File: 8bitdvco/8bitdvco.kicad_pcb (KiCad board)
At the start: 2 copper layers, 87.4 x 66.8 mm, 30 parts, among them J1 PWR_IN, J2 SPI, J3 DISP, J4 UART, J5 THERM, J6 FAN, J7 HEAT, SW1 SW_RST, SW2 SW_STOP_MODE, SW3 SW_START_SET, U1 ATmega328P-PU, Y1 16MHz

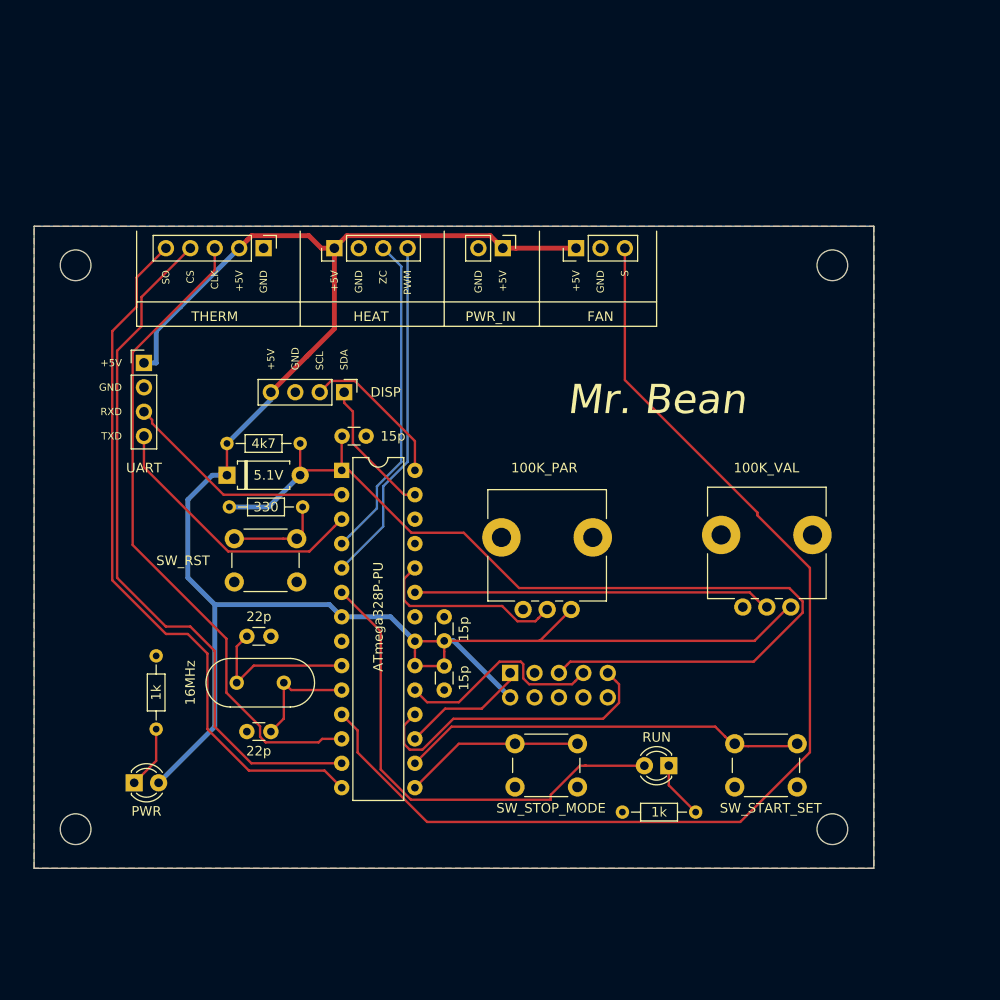
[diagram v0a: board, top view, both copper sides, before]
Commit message: done without errors and warnings
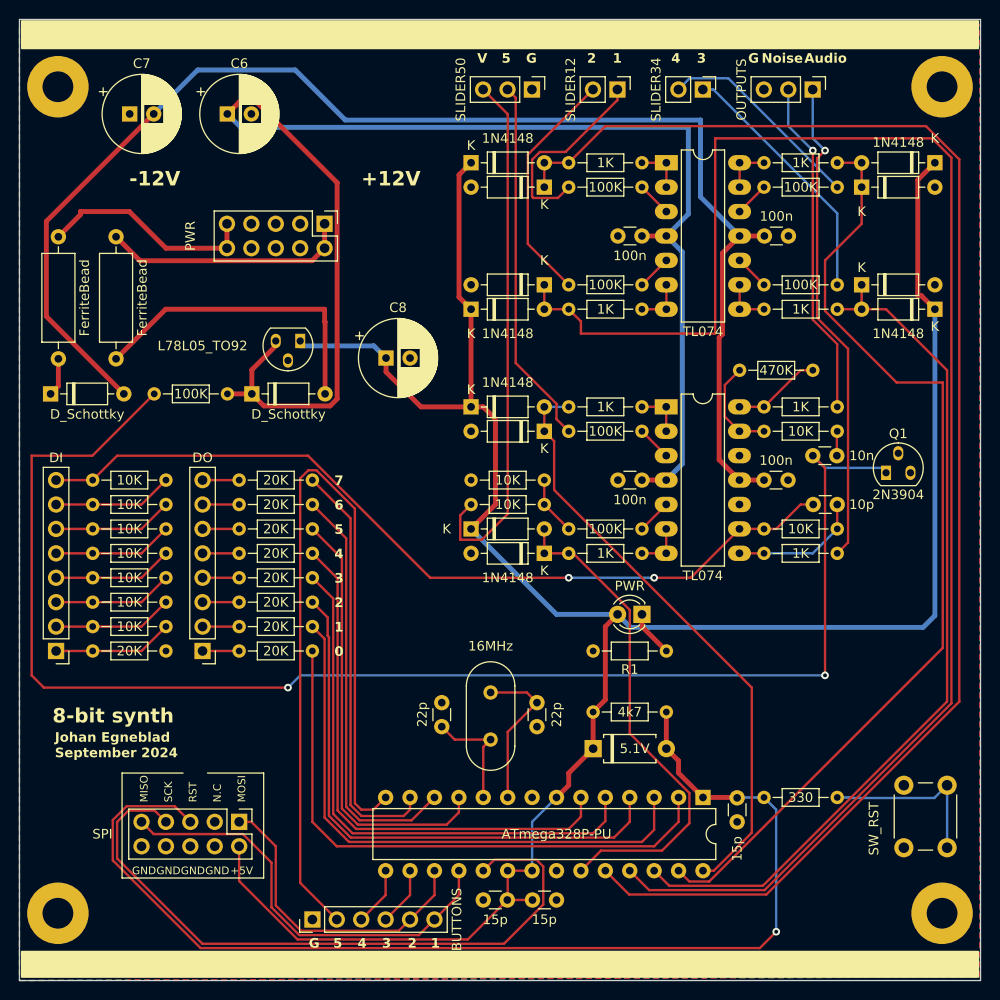
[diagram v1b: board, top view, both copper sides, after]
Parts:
- removed the REF** at (43.9, 98.6)
- removed the REF** at (43.9, 39.9)
- removed the REF** at (122.7, 98.6)
- removed the REF** at (122.7, 39.9)
- removed RV1: 100K_VAL, Potentiometer_THT:Potentiometer_Alps_RK09L_Single_Vertical
- removed RV2: 100K_PAR, Potentiometer_THT:Potentiometer_Alps_RK09L_Single_Vertical
- removed SW2: SW_STOP_MODE, Button_Switch_THT:SW_PUSH_6mm_H4.3mm
- removed SW3: SW_START_SET, Button_Switch_THT:SW_PUSH_6mm_H4.3mm
- added C10: 100n, Capacitor_THT:C_Disc_D3.0mm_W1.6mm_P2.50mm, F.Cu at (118.1, 62.2)
- added C11: 100n, Capacitor_THT:C_Disc_D3.0mm_W1.6mm_P2.50mm, F.Cu at (100.4, 36.8)
- added C12: 100n, Capacitor_THT:C_Disc_D3.0mm_W1.6mm_P2.50mm, F.Cu at (118.1, 36.8)
- added C13: 10p, Capacitor_THT:C_Disc_D3.0mm_W1.6mm_P2.50mm, F.Cu at (120.7, 64.8)
- added C14: 10n, Capacitor_THT:C_Disc_D3.0mm_W1.6mm_P2.50mm, F.Cu at (123.2, 59.7)
- added C6: C_Polarized, Capacitor_THT:CP_Radial_D8.0mm_P2.50mm, F.Cu at (59.7, 24.1)
- added C7: C_Polarized, Capacitor_THT:CP_Radial_D8.0mm_P2.50mm, F.Cu at (49.6, 24.1)
- added C8: C_Polarized, Capacitor_THT:CP_Radial_D8.0mm_P2.50mm, F.Cu at (76.2, 49.5)
- added C9: 100n, Capacitor_THT:C_Disc_D3.0mm_W1.6mm_P2.50mm, F.Cu at (100.4, 62.2)
- added D10: 1N4148, Diode_THT:D_DO-35_SOD27_P7.62mm_Horizontal, F.Cu at (125.7, 41.9)
- added D11: 1N4148, Diode_THT:D_DO-35_SOD27_P7.62mm_Horizontal, F.Cu at (133.3, 29.2)
- added D12: 1N4148, Diode_THT:D_DO-35_SOD27_P7.62mm_Horizontal, F.Cu at (125.7, 31.8)
- added D13: 1N4148, Diode_THT:D_DO-35_SOD27_P7.62mm_Horizontal, F.Cu at (85.1, 54.6)
- added D14: 1N4148, Diode_THT:D_DO-35_SOD27_P7.62mm_Horizontal, F.Cu at (92.7, 57.1)
- added D15: 1N4148, Diode_THT:D_DO-35_SOD27_P7.62mm_Horizontal, F.Cu at (85.1, 67.3)
- added D16: 1N4148, Diode_THT:D_DO-35_SOD27_P7.62mm_Horizontal, F.Cu at (92.7, 69.8)
- added D4: D_Schottky, Diode_THT:D_DO-35_SOD27_P7.62mm_Horizontal, F.Cu at (62.3, 53.3)
- added D5: D_Schottky, Diode_THT:D_DO-35_SOD27_P7.62mm_Horizontal, F.Cu at (41.3, 53.3)
- added D6: 1N4148, Diode_THT:D_DO-35_SOD27_P7.62mm_Horizontal, F.Cu at (92.7, 31.8)
- added D7: 1N4148, Diode_THT:D_DO-35_SOD27_P7.62mm_Horizontal, F.Cu at (85.1, 44.5)
- added D8: 1N4148, Diode_THT:D_DO-35_SOD27_P7.62mm_Horizontal, F.Cu at (92.7, 41.9)
- added D9: 1N4148, Diode_THT:D_DO-35_SOD27_P7.62mm_Horizontal, F.Cu at (133.3, 44.5)
- added FB1: FerriteBead, Resistor_THT:R_Axial_DIN0309_L9.0mm_D3.2mm_P12.70mm_Horizontal, F.Cu at (48.1, 49.6)
- added FB2: FerriteBead, Resistor_THT:R_Axial_DIN0309_L9.0mm_D3.2mm_P12.70mm_Horizontal, F.Cu at (42.1, 49.6)
- added J8: OUTPUTS, Connector_PinHeader_2.54mm:PinHeader_1x03_P2.54mm_Vertical, F.Cu at (120.6, 21.6)
- added J9: BUTTONS, Connector_PinHeader_2.54mm:PinHeader_1x06_P2.54mm_Vertical, F.Cu at (68.6, 108.0)
- added Q1: 2N3904, Package_TO_SOT_THT:TO-92_Inline, F.Cu at (128.3, 61.0)
- added R10: 10K, Resistor_THT:R_Axial_DIN0204_L3.6mm_D1.6mm_P7.62mm_Horizontal, F.Cu at (53.3, 62.2)
- added R11: 20K, Resistor_THT:R_Axial_DIN0204_L3.6mm_D1.6mm_P7.62mm_Horizontal, F.Cu at (53.3, 80.0)
- added R12: 1K, Resistor_THT:R_Axial_DIN0204_L3.6mm_D1.6mm_P7.62mm_Horizontal, F.Cu at (102.9, 29.2)
- added R13: 100K, Resistor_THT:R_Axial_DIN0204_L3.6mm_D1.6mm_P7.62mm_Horizontal, F.Cu at (95.2, 31.8)
- added R14: 20K, Resistor_THT:R_Axial_DIN0204_L3.6mm_D1.6mm_P7.62mm_Horizontal, F.Cu at (68.6, 80.0)
- added R15: 20K, Resistor_THT:R_Axial_DIN0204_L3.6mm_D1.6mm_P7.62mm_Horizontal, F.Cu at (68.6, 77.5)
- added R16: 20K, Resistor_THT:R_Axial_DIN0204_L3.6mm_D1.6mm_P7.62mm_Horizontal, F.Cu at (68.6, 74.9)
- added R17: 20K, Resistor_THT:R_Axial_DIN0204_L3.6mm_D1.6mm_P7.62mm_Horizontal, F.Cu at (68.6, 72.4)
- added R18: 20K, Resistor_THT:R_Axial_DIN0204_L3.6mm_D1.6mm_P7.62mm_Horizontal, F.Cu at (68.6, 69.8)
- added R19: 20K, Resistor_THT:R_Axial_DIN0204_L3.6mm_D1.6mm_P7.62mm_Horizontal, F.Cu at (68.6, 67.3)
- added R20: 20K, Resistor_THT:R_Axial_DIN0204_L3.6mm_D1.6mm_P7.62mm_Horizontal, F.Cu at (68.6, 64.8)
- added R21: 20K, Resistor_THT:R_Axial_DIN0204_L3.6mm_D1.6mm_P7.62mm_Horizontal, F.Cu at (68.6, 62.2)
- added R22: 100K, Resistor_THT:R_Axial_DIN0204_L3.6mm_D1.6mm_P7.62mm_Horizontal, F.Cu at (95.2, 41.9)
- added R23: 1K, Resistor_THT:R_Axial_DIN0204_L3.6mm_D1.6mm_P7.62mm_Horizontal, F.Cu at (102.9, 44.5)
- added R24: 1K, Resistor_THT:R_Axial_DIN0204_L3.6mm_D1.6mm_P7.62mm_Horizontal, F.Cu at (115.6, 44.5)
- added R25: 1K, Resistor_THT:R_Axial_DIN0204_L3.6mm_D1.6mm_P7.62mm_Horizontal, F.Cu at (115.6, 29.2)
- added R26: 100K, Resistor_THT:R_Axial_DIN0204_L3.6mm_D1.6mm_P7.62mm_Horizontal, F.Cu at (123.2, 41.9)
- added R27: 100K, Resistor_THT:R_Axial_DIN0204_L3.6mm_D1.6mm_P7.62mm_Horizontal, F.Cu at (123.2, 31.8)
- added R28: 1K, Resistor_THT:R_Axial_DIN0204_L3.6mm_D1.6mm_P7.62mm_Horizontal, F.Cu at (102.9, 54.6)
- added R29: 1K, Resistor_THT:R_Axial_DIN0204_L3.6mm_D1.6mm_P7.62mm_Horizontal, F.Cu at (102.9, 69.8)
- added R30: 100K, Resistor_THT:R_Axial_DIN0204_L3.6mm_D1.6mm_P7.62mm_Horizontal, F.Cu at (95.2, 57.1)
- added R31: 100K, Resistor_THT:R_Axial_DIN0204_L3.6mm_D1.6mm_P7.62mm_Horizontal, F.Cu at (95.2, 67.3)
- added R32: 10K, Resistor_THT:R_Axial_DIN0204_L3.6mm_D1.6mm_P7.62mm_Horizontal, F.Cu at (92.7, 64.8)
- added R33: 10K, Resistor_THT:R_Axial_DIN0204_L3.6mm_D1.6mm_P7.62mm_Horizontal, F.Cu at (85.1, 62.2)
- added R34: 10K, Resistor_THT:R_Axial_DIN0204_L3.6mm_D1.6mm_P7.62mm_Horizontal, F.Cu at (115.6, 67.3)
- added R35: 1K, Resistor_THT:R_Axial_DIN0204_L3.6mm_D1.6mm_P7.62mm_Horizontal, F.Cu at (115.6, 69.8)
- added R36: 1K, Resistor_THT:R_Axial_DIN0204_L3.6mm_D1.6mm_P7.62mm_Horizontal, F.Cu at (115.6, 54.6)
- added R37: 470K, Resistor_THT:R_Axial_DIN0204_L3.6mm_D1.6mm_P7.62mm_Horizontal, F.Cu at (113.0, 50.8)
- added R38: 10K, Resistor_THT:R_Axial_DIN0204_L3.6mm_D1.6mm_P7.62mm_Horizontal, F.Cu at (123.2, 57.1)
- added R39: 100K, Resistor_THT:R_Axial_DIN0204_L3.6mm_D1.6mm_P7.62mm_Horizontal, F.Cu at (52.1, 53.3)
- added R5: 10K, Resistor_THT:R_Axial_DIN0204_L3.6mm_D1.6mm_P7.62mm_Horizontal, F.Cu at (53.3, 74.9)
- added R6: 10K, Resistor_THT:R_Axial_DIN0204_L3.6mm_D1.6mm_P7.62mm_Horizontal, F.Cu at (53.3, 72.4)
- added R7: 10K, Resistor_THT:R_Axial_DIN0204_L3.6mm_D1.6mm_P7.62mm_Horizontal, F.Cu at (53.3, 69.8)
- added R8: 10K, Resistor_THT:R_Axial_DIN0204_L3.6mm_D1.6mm_P7.62mm_Horizontal, F.Cu at (53.3, 67.3)
- added R9: 10K, Resistor_THT:R_Axial_DIN0204_L3.6mm_D1.6mm_P7.62mm_Horizontal, F.Cu at (53.3, 64.8)
- added REF**: MountingHole_3.2mm_M3_Pad, MountingHole:MountingHole_3.2mm_M3_Pad, F.Cu at (42.1, 107.3)
- added REF**: MountingHole_3.2mm_M3_Pad, MountingHole:MountingHole_3.2mm_M3_Pad, F.Cu at (134.1, 107.3)
- added REF**: MountingHole_3.2mm_M3_Pad, MountingHole:MountingHole_3.2mm_M3_Pad, F.Cu at (134.1, 21.3)
- added REF**: MountingHole_3.2mm_M3_Pad, MountingHole:MountingHole_3.2mm_M3_Pad, F.Cu at (42.1, 21.3)
- added U2: L78L05_TO92, Package_TO_SOT_THT:TO-92_Inline, F.Cu at (67.3, 48.3)
- added U3: TL074, Package_DIP:DIP-14_W7.62mm_LongPads, F.Cu at (105.4, 29.2)
- added U4: TL074, Package_DIP:DIP-14_W7.62mm_LongPads, F.Cu at (105.4, 54.6)
- D3: value RUN -> 1N4148; footprint LED_THT:LED_D3.0mm -> Diode_THT:D_DO-35_SOD27_P7.62mm_Horizontal
- J1: value PWR_IN -> DO; footprint Connector_PinHeader_2.54mm:PinHeader_1x02_P2.54mm_Vertical -> Connector_PinHeader_2.54mm:PinHeader_1x08_P2.54mm_Vertical
- J2: moved to F.Cu
- J3: value DISP -> PWR; footprint Connector_PinHeader_2.54mm:PinHeader_1x04_P2.54mm_Vertical -> Connector_PinHeader_2.54mm:PinHeader_2x05_P2.54mm_Vertical
- J4: value UART -> DI; footprint Connector_PinHeader_2.54mm:PinHeader_1x04_P2.54mm_Vertical -> Connector_PinHeader_2.54mm:PinHeader_1x08_P2.54mm_Vertical
- J5: value THERM -> SLIDER12; footprint Connector_PinHeader_2.54mm:PinHeader_1x05_P2.54mm_Vertical -> Connector_PinHeader_2.54mm:PinHeader_1x02_P2.54mm_Vertical
- J6: value FAN -> SLIDER34; footprint Connector_PinHeader_2.54mm:PinHeader_1x03_P2.54mm_Vertical -> Connector_PinHeader_2.54mm:PinHeader_1x02_P2.54mm_Vertical
- J7: value HEAT -> SLIDER50; footprint Connector_PinHeader_2.54mm:PinHeader_1x04_P2.54mm_Vertical -> Connector_PinHeader_2.54mm:PinHeader_1x03_P2.54mm_Vertical
- R4: value 1k -> 10K
- moved SW1 78.5 mm to (134.6, 94.0), turned to -90 degrees
- moved D3 66.0 mm to (85.1, 29.2), turned to 0 degrees
- moved R3 63.3 mm to (123.2, 95.2)
- moved R4 58.4 mm to (53.3, 77.5)
- moved C5 55.7 mm to (112.8, 97.8), turned to 90 degrees
- moved D1 55.7 mm to (102.9, 76.2), turned to 180 degrees
- moved R1 53.7 mm to (105.4, 80.0), turned to 180 degrees
- moved J1 52.3 mm to (57.1, 80.0), turned to 180 degrees
- moved U1 50.7 mm to (109.2, 95.2), turned to -90 degrees
- moved D2 47.5 mm to (97.8, 90.2)
- moved R2 47.2 mm to (97.8, 86.4)
- moved J5 40.3 mm to (100.3, 21.6)
- moved J2 32.2 mm to (61.0, 97.8)
- moved C2 31.7 mm to (94.0, 105.9), turned to 180 degrees
- moved J4 31.3 mm to (41.9, 80.0), turned to 180 degrees
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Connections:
- net Net-(C3-Pad2) renamed /XTAL1
- net Net-(C4-Pad1) renamed /XTAL2
- D3 pad 1: Net-(D3-Pad1) -> +5V
- D3 pad 2: /LED_RUNNING -> /A1
- J1 pad 1: +5V -> Net-(J1-Pin_1)
- J1 pad 2: GND -> Net-(J1-Pin_2)
- J2 pad 3: Net-(J2-Pad3) -> unconnected-(J2-Pin_3-Pad3)
- J3 pad 1: /SDA -> Net-(J3-Pin_1)
- J3 pad 2: /SCL -> Net-(J3-Pin_1)
- J3 pad 4: +5V -> GND
- J4 pad 1: +5V -> Net-(J4-Pin_1)
- J4 pad 2: GND -> Net-(J4-Pin_2)
- J4 pad 3: /RXD -> Net-(J4-Pin_3)
- J4 pad 4: /TXD -> Net-(J4-Pin_4)
- J5 pad 1: GND -> /SLIDER1
- J5 pad 2: +5V -> /SLIDER2
- J6 pad 1: +5V -> /SLIDER3
- J6 pad 2: GND -> /SLIDER4
- J7 pad 1: +5V -> GND
- J7 pad 2: GND -> /SLIDER5
- J7 pad 3: /ZERO_CROSS -> /VOCT
- R4 pad 1: Net-(D3-Pad1) -> Net-(J4-Pin_1)
- R4 pad 2: GND -> Net-(J4-Pin_2)
- U1 pad 11: /FAN_S -> /DAC5
- U1 pad 12: /CLK -> /DAC6
- U1 pad 13: /CS -> /DAC7
- U1 pad 14: /SO -> /S5
- U1 pad 15: /SW_STOP_MODE -> /S4
- U1 pad 16: /SW_START_SET -> /S3
- U1 pad 2: /RXD -> /DAC0
- U1 pad 25: Net-(U1-Pad25) -> /A2
- U1 pad 26: Net-(U1-Pad26) -> /A3
- U1 pad 27: /SDA -> /A4
- U1 pad 28: /SCL -> /A5
- U1 pad 3: /TXD -> /DAC1
- U1 pad 4: /ZERO_CROSS -> /DAC2
- U1 pad 5: /TRIAC_GATE -> /DAC3
- U1 pad 6: /LED_RUNNING -> /DAC4
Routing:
- net /A2: track 0.00 -> 167.0 mm
- net Net-(Q1-E): track 0.00 -> 153.4 mm, vias 0 -> 2
- net +12V: track 0.00 -> 148.8 mm
- net -12V: track 0.00 -> 144.1 mm
- net /A1: track 20.1 -> 151.3 mm
- net /FAN_S: track 118.1 -> 0.00 mm
- net /A4: track 0.00 -> 100.5 mm
- net /A3: track 0.00 -> 90.1 mm
- net /S5: track 0.00 -> 89.8 mm
- net /DAC: track 0.00 -> 88.3 mm, vias 0 -> 2
- net /SO: track 74.3 -> 0.00 mm
- net /CS: track 73.4 -> 0.00 mm
- net /CLK: track 68.7 -> 0.00 mm
- net /A5: track 0.00 -> 62.5 mm
- net /DAC0: track 0.00 -> 60.5 mm
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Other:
- board size 87.4 x 66.8 mm -> 100 x 100 mm
- net class Default removed
- board text added: "+12V"
- board text added: "-12V"
- board text added: "0"
- board text added: "1"
- board text added: "2"
- board text added: "3"
- board text added: "4"
- board text added: "5"
- board text added: "6"
- board text added: "7"
- board text added: "8-bit synth"
- board text added: "Audio"
- board text added: "G"
- board text added: "Johan Egneblad September 2024"
- board text added: "Noise"
- board text added: "V"
- board text removed: "CLK"
- board text removed: "CS"
- board text removed: "Mr. Bean"
- board text removed: "PWM"
- board text removed: "RXD"
- board text removed: "S"
- board text removed: "SCL"
- board text removed: "SDA"
- board text removed: "SO"
- board text removed: "TXD"
- board text removed: "ZC"
